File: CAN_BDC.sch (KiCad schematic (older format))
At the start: 28 parts, among them P1 CONN_01X02, P2 CONN_01X05, P3 CONN_01X02, P4 CONN_01X02, P5 CONN_01X02, P6 CONN_01X02, P7 CONN_01X04, U1 PSD2CAN, U2 SN65HVD232D, U3 POLOLU_A4988, U4 STM32F042G4U6, U5 MC33063

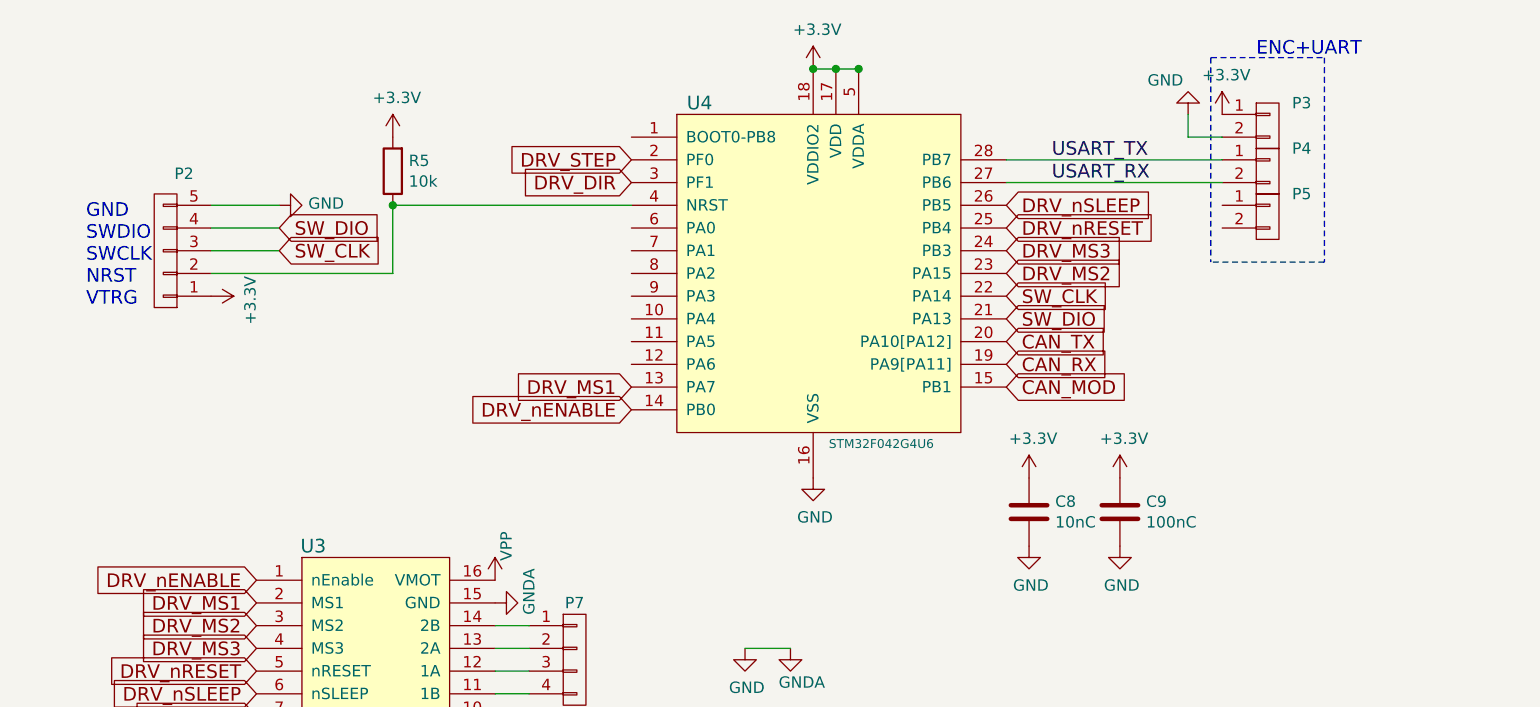
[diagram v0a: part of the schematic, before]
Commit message: Layout improve
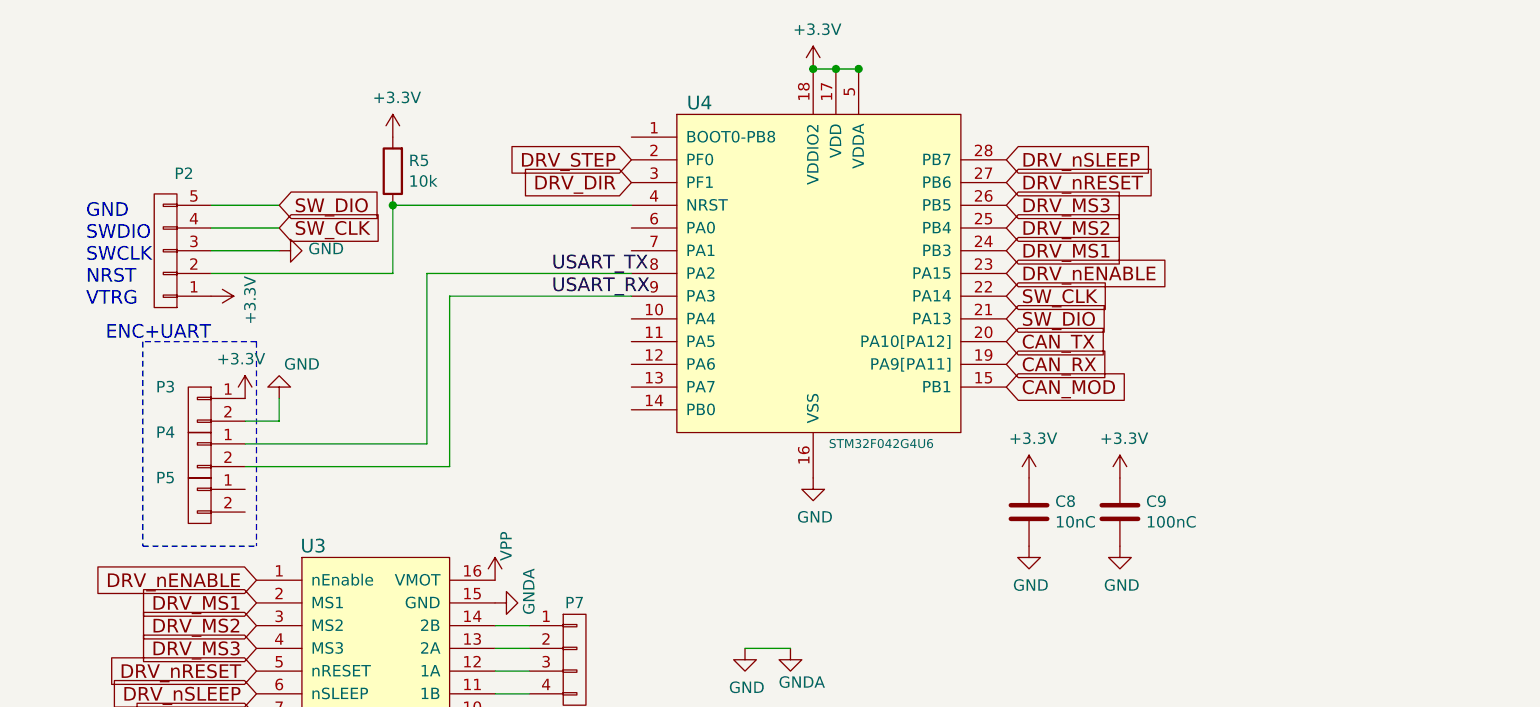
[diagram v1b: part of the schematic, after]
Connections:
- net DRV_MS1: now also U4.24 (PB3); no longer U4.13 (PA7)
- net DRV_MS2: now also U4.25 (PB4); no longer U4.23 (PA15)
- net DRV_MS3: now also U4.26 (PB5); no longer U4.24 (PB3)
- net DRV_nENABLE: now also U4.23 (PA15); no longer U4.14 (PB0)
- net DRV_nRESET: now also U4.27 (PB6); no longer U4.25 (PB4)
- net DRV_nSLEEP: now also U4.28 (PB7); no longer U4.26 (PB5)
- net GND: now also P2.3 (P3); no longer P2.5 (P5)
- net SW_CLK: now also P2.4 (P4); no longer P2.3 (P3)
- net SW_DIO: now also P2.5 (P5); no longer P2.4 (P4)
- net USART_RX: now also U4.9 (PA3); no longer U4.27 (PB6)
- net USART_TX: now also U4.8 (PA2); no longer U4.28 (PB7)
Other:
- moved on the sheet: P3, P4, P5
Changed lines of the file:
@@
 	1    0    0    -1
 $EndComp
-Text GLabel 1900 1800 2    60   Input ~ 0
+Text GLabel 1900 1700 2    60   Input ~ 0
 SW_CLK
 Text GLabel 5100 2000 2    60   Input ~ 0
 SW_CLK
-Text GLabel 1900 1700 2    60   Input ~ 0
+Text GLabel 1900 1600 2    60   Input ~ 0
 SW_DIO
 Text GLabel 5100 2100 2    60   Input ~ 0
@@
 L GND #PWR011
 U 1 1 571ACD79
-P 5900 1200
-F 0 "#PWR011" H 5900 950 50  0001 C CNN
-F 1 "GND" H 6000 1050 50  0000 C CNN
-F 2 "" H 5900 1200 50  0000 C CNN
-F 3 "" H 5900 1200 50  0000 C CNN
-	1    5900 1200
-	-1   0    0    1
-$EndComp
-Text Label 5300 1400 0    60   ~ 0
-USART_TX
-Text Label 5300 1500 0    60   ~ 0
-USART_RX
+P 1900 2450
+F 0 "#PWR011" H 1900 2200 50  0001 C CNN
+F 1 "GND" H 2000 2300 50  0000 C CNN
+F 2 "" H 1900 2450 50  0000 C CNN
+F 3 "" H 1900 2450 50  0000 C CNN
+	1    1900 2450
+	1    0    0    1
+$EndComp
 $Comp
 L +3.3V #PWR012
@@
 L +3.3V #PWR013
 U 1 1 57F6DF04
-P 6050 1200
-F 0 "#PWR013" H 6050 1050 50  0001 C CNN
-F 1 "+3.3V" H 6068 1373 50  0000 C CNN
-F 2 "" H 6050 1200 50  0000 C CNN
-F 3 "" H 6050 1200 50  0000 C CNN
-	1    6050 1200
-	1    0    0    -1
+P 1750 2450
+F 0 "#PWR013" H 1750 2300 50  0001 C CNN
+F 1 "+3.3V" H 1768 2623 50  0000 C CNN
+F 2 "" H 1750 2450 50  0000 C CNN
+F 3 "" H 1750 2450 50  0000 C CNN
+	1    1750 2450
+	-1   0    0    -1
 $EndComp
 $Comp
@@
 L GND #PWR015
 U 1 1 57056C83
-P 1900 1600
-F 0 "#PWR015" H 1900 1350 50  0001 C CNN
-F 1 "GND" V 1908 1472 50  0000 R CNN
-F 2 "" H 1900 1600 50  0000 C CNN
-F 3 "" H 1900 1600 50  0000 C CNN
-	1    1900 1600
+P 1900 1800
+F 0 "#PWR015" H 1900 1550 50  0001 C CNN
+F 1 "GND" V 1908 1672 50  0000 R CNN
+F 2 "" H 1900 1800 50  0000 C CNN
+F 3 "" H 1900 1800 50  0000 C CNN
+	1    1900 1800
 	0    -1   -1   0
 $EndComp
@@
 L CONN_01X02 P3
 U 1 1 57FD66CE
-P 6250 1250
-F 0 "P3" H 6400 1350 50  0000 C CNN
-F 1 "CONN_01X02" V 6124 1106 50  0001 R CNN
-F 2 "Pin_Headers:Pin_Header_Straight_1x02_Pitch2.00mm" H 6250 1250 50  0001 C CNN
-F 3 "" H 6250 1250 50  0000 C CNN
-	1    6250 1250
-	1    0    0    -1
+P 1550 2500
+F 0 "P3" H 1700 2600 50  0000 C CNN
+F 1 "CONN_01X02" V 1424 2356 50  0001 R CNN
+F 2 "Pin_Headers:Pin_Header_Straight_1x02_Pitch2.00mm" H 1550 2500 50  0001 C CNN
+F 3 "" H 1550 2500 50  0000 C CNN
+	1    1550 2500
+	-1   0    0    -1
 $EndComp
 $Comp
 L CONN_01X02 P4
 U 1 1 57FD69A3
-P 6250 1450
-F 0 "P4" H 6400 1550 50  0000 C CNN
-F 1 "CONN_01X02" V 6124 1306 50  0001 R CNN
-F 2 "Pin_Headers:Pin_Header_Straight_1x02_Pitch2.00mm" H 6250 1450 50  0001 C CNN
-F 3 "" H 6250 1450 50  0000 C CNN
-	1    6250 1450
-	1    0    0    -1
+P 1550 2700
+F 0 "P4" H 1700 2800 50  0000 C CNN
+F 1 "CONN_01X02" V 1424 2556 50  0001 R CNN
+F 2 "Pin_Headers:Pin_Header_Straight_1x02_Pitch2.00mm" H 1550 2700 50  0001 C CNN
+F 3 "" H 1550 2700 50  0000 C CNN
+	1    1550 2700
+	-1   0    0    -1
 $EndComp
 $Comp
@@
 	3400 5200 4550 5200
 Wire Wire Line
-	5900 1300 6050 1300
-Wire Wire Line
-	5900 1300 5900 1200
+	1900 2550 1750 2550
+Wire Wire Line
+	1900 2550 1900 2450
 Connection ~ 2400 1600
 Wire Wire Line
@@
 L CONN_01X02 P5
 U 1 1 58059EA3
-P 6250 1650
-F 0 "P5" H 6400 1750 50  0000 C CNN
-F 1 "CONN_01X02" V 6124 1506 50  0001 R CNN
-F 2 "Pin_Headers:Pin_Header_Straight_1x02_Pitch2.00mm" H 6250 1650 50  0001 C CNN
-F 3 "" H 6250 1650 50  0000 C CNN
-	1    6250 1650
-	1    0    0    -1
+P 1550 2900
+F 0 "P5" H 1700 3000 50  0000 C CNN
+F 1 "CONN_01X02" V 1424 2756 50  0001 R CNN
+F 2 "Pin_Headers:Pin_Header_Straight_1x02_Pitch2.00mm" H 1550 2900 50  0001 C CNN
+F 3 "" H 1550 2900 50  0000 C CNN
+	1    1550 2900
+	-1   0    0    -1
 $EndComp
 Wire Notes Line
-	6000 950  6000 1850
+	1800 2200 1800 3100
 Wire Notes Line
-	6000 950  6500 950
+	1800 2200 1300 2200
 Wire Notes Line
-	6500 950  6500 1850
+	1300 2200 1300 3100
 Wire Notes Line
-	6500 1850 6000 1850
-Text Notes 6200 950  0    60   ~ 0
+	1300 3100 1800 3100
+Text Notes 1600 2200 2    60   ~ 0
 ENC+UART
 $Comp
@@
 Connection ~ 4250 5550
 Wire Wire Line
-	5100 1400 6050 1400
-Wire Wire Line
-	6050 1500 5100 1500
-Wire Wire Line
 	2400 1600 3450 1600
 $Comp
@@
 	-1   0    0    1
 $EndComp
-Text GLabel 3450 2500 0    60   Input ~ 0
+Text GLabel 5100 1900 2    60   Input ~ 0
 DRV_nENABLE
-Text GLabel 3450 2400 0    60   Input ~ 0
+Text GLabel 5100 1800 2    60   Input ~ 0
 DRV_MS1
-Text GLabel 5100 1900 2    60   Input ~ 0
+Text GLabel 5100 1700 2    60   Input ~ 0
 DRV_MS2
-Text GLabel 5100 1800 2    60   Input ~ 0
+Text GLabel 5100 1600 2    60   Input ~ 0
 DRV_MS3
-Text GLabel 5100 1700 2    60   Input ~ 0
+Text GLabel 5100 1500 2    60   Input ~ 0
 DRV_nRESET
-Text GLabel 5100 1600 2    60   Input ~ 0
+Text GLabel 5100 1400 2    60   Input ~ 0
 DRV_nSLEEP
 Text GLabel 3450 1400 0    60   Input ~ 0
@@
 Text Notes 8350 2300 0    60   ~ 0
 WYPROWADZ BOOT\nODLACZENIE PRZETWORNICY\n3V3 i przetwornica na raz\n
+Text Label 3100 2000 0    60   ~ 0
+USART_RX
+Text Label 3100 1900 0    60   ~ 0
+USART_TX
+Wire Wire Line
+	3450 2000 2650 2000
+Wire Wire Line
+	2650 2000 2650 2750
+Wire Wire Line
+	2650 2750 1750 2750
+Wire Wire Line
+	3450 1900 2550 1900
+Wire Wire Line
+	2550 1900 2550 2650
+Wire Wire Line
+	2550 2650 1750 2650
 $EndSCHEMATC
